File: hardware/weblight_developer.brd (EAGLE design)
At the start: 40.6 x 12 mm, 14 parts, among them U1 ATtiny85-20SU

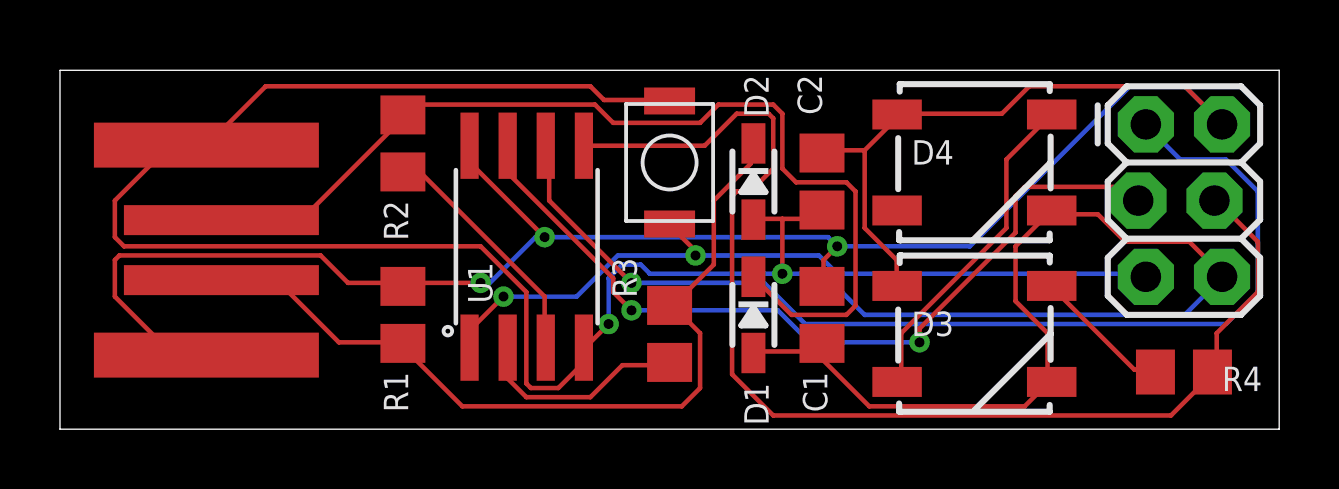
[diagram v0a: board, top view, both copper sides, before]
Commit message: osh3 rc1
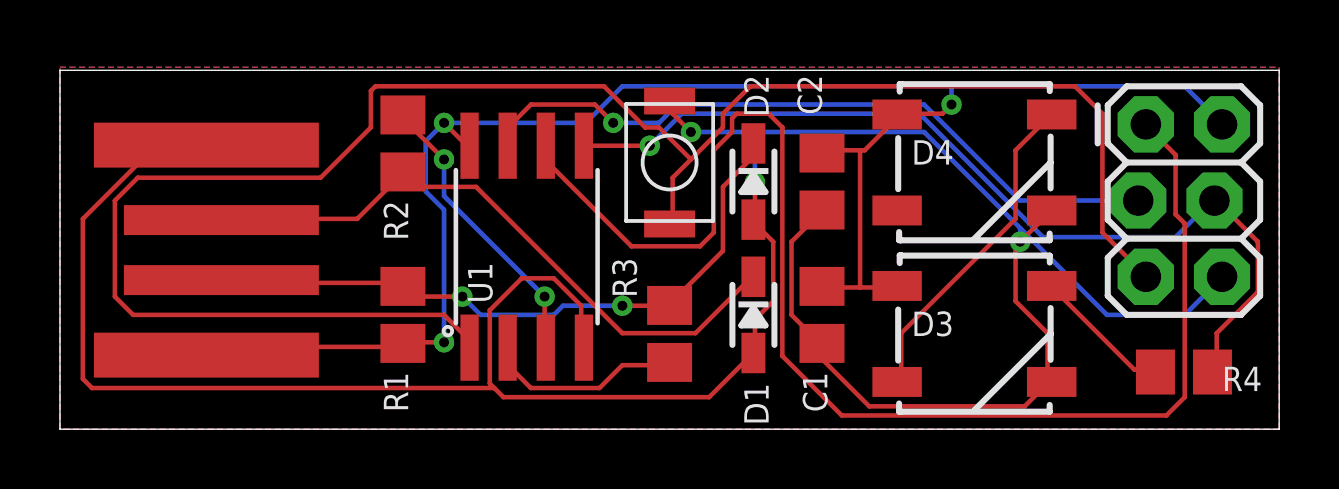
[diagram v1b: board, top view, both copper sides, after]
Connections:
- net USB_D_MINUS_RAW: now also R1.1; no longer R1.2
- net USB_D_PLUS: now also R2.1; no longer R2.2
- net USB_D_PLUS_RAW: now also R2.2; no longer R2.1
- net VCC: now also R1.2; no longer R1.1
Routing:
- net RESET: track 25.9 -> 62.3 mm, vias 2 -> 0
- net VCC: track 71.6 -> 56.9 mm
- net USB_D_PLUS_RAW: track 33.5 -> 21.4 mm
- net MOSI/DIN_RAW: track 40.4 -> 30.7 mm, vias 0 -> 1
- net MISO: track 35.7 -> 45.3 mm, vias 1 -> 0
- net USB_D_MINUS_RAW: track 27.8 -> 22.2 mm, vias 0 -> 2
- net SCK: track 27.9 -> 23.8 mm, vias 2 -> 1
- net GND: track 95.8 -> 93.3 mm, vias 2 -> 3
- net USB_D_PLUS: track 8.19 -> 9.73 mm, vias 0 -> 2
- net USB_D_MINUS: track 7.17 -> 6.65 mm
- added copper zone on layer 1, net GND
- added copper zone on layer 16, net GND
